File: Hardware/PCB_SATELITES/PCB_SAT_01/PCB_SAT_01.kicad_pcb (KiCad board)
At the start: 4 copper layers, 60 x 79 mm, 17 parts, among them IC1 OPT3001DNPRQ1, IC2 OPT3001DNPRQ1, IC3 OPT3001DNPRQ1, IC4 OPT3001DNPRQ1, J1 MTJ-88ARX1-FSM-LG

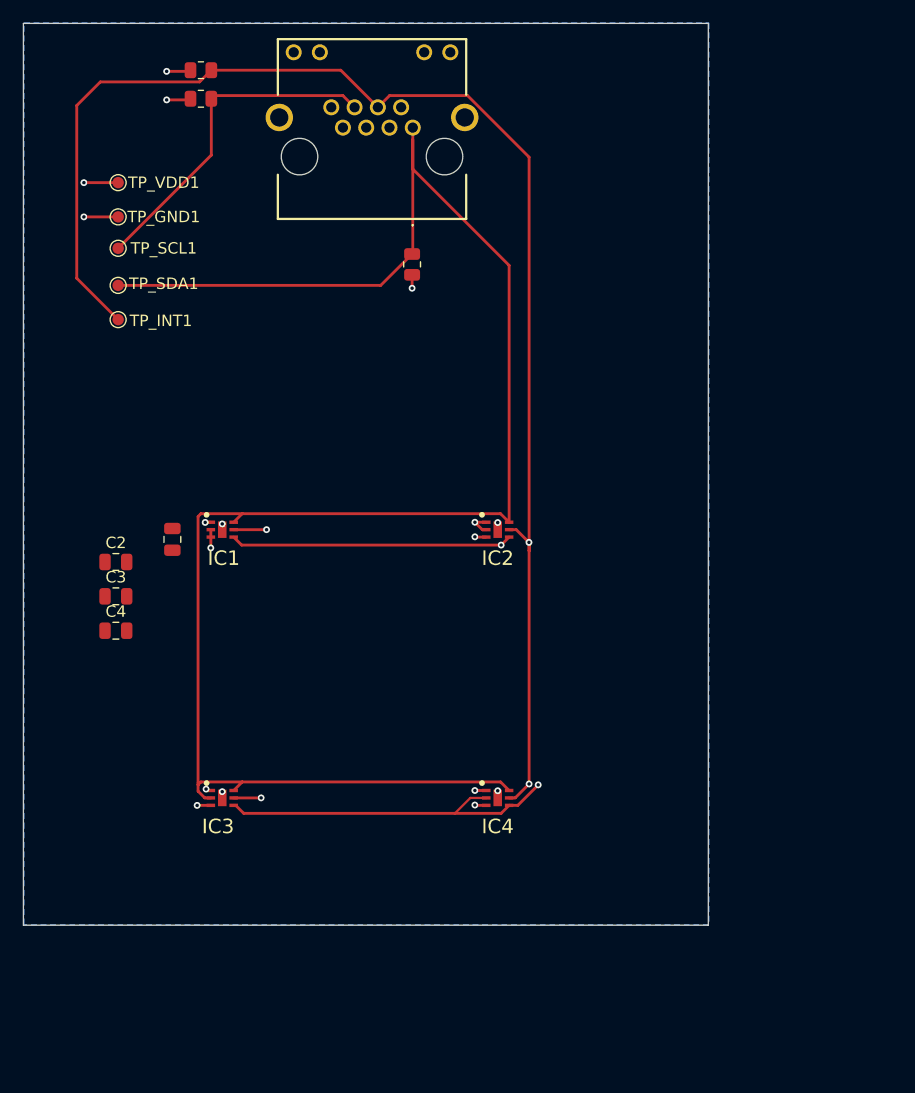
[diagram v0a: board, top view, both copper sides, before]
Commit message: actualizacion pcb satelite 1
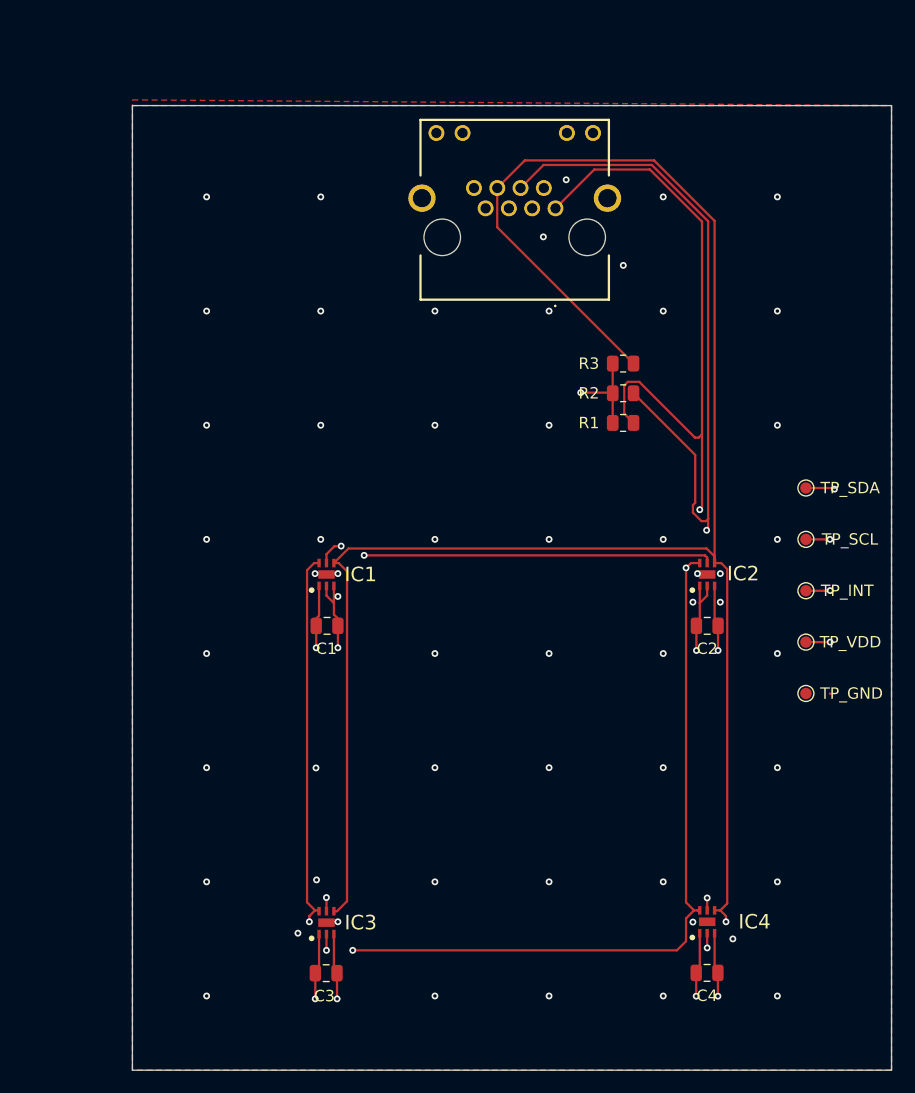
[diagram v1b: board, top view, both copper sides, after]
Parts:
- removed TP_GND1, TP_INT1, TP_SCL1, TP_SDA1, TP_VDD1: TestPoint, TestPoint:TestPoint_Pad_D1.0mm
- added TP_GND: TestPoint, TestPoint:TestPoint_Pad_D1.0mm, F.Cu at (142.5, 108.5)
- added TP_INT: TestPoint, TestPoint:TestPoint_Pad_D1.0mm, F.Cu at (142.5, 99.5)
- added TP_SCL: TestPoint, TestPoint:TestPoint_Pad_D1.0mm, F.Cu at (142.5, 95.0)
- added TP_SDA: TestPoint, TestPoint:TestPoint_Pad_D1.0mm, F.Cu at (142.5, 90.5)
- added TP_VDD: TestPoint, TestPoint:TestPoint_Pad_D1.0mm, F.Cu at (142.5, 104.0)
- moved C4 59.8 mm to (133.8, 133.0)
- moved C2 52.1 mm to (133.9, 102.6)
- moved R2 46.6 mm to (126.5, 82.2)
- moved R3 43.7 mm to (126.5, 79.6)
- moved C3 37.8 mm to (100.5, 133.0)
- moved R1 23.1 mm to (126.5, 84.8), turned to 0 degrees
- moved IC4 21.3 mm to (133.8, 128.5), turned to 90 degrees
- moved IC2 18.8 mm to (133.8, 98.1), turned to 90 degrees
- moved C1 15.5 mm to (100.5, 102.6), turned to 0 degrees
- moved J1 14.4 mm to (120.6, 66.0)
- moved IC3 14.2 mm to (100.5, 128.6), turned to 90 degrees
- moved IC1 9.94 mm to (100.5, 98.1), turned to 90 degrees
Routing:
- net /SCL: track 160.9 -> 221.8 mm, vias 2 -> 3
- net /INT: track 177.9 -> 232.2 mm, vias 4 -> 6
- net /SDA: track 158.3 -> 181.2 mm, vias 0 -> 6
- net VDD: track 12.7 -> 34.2 mm, vias 8 -> 6
- net GND: track 10.1 -> 24.0 mm, vias 9 -> 61
- added copper zone on In1.Cu, net (none)
- added copper zone on F.Cu, net GND
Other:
- board size 60 x 79 mm -> 66.5 x 84.5 mm
- board text removed: "OPT3001DNPRQ1"
- board text removed: "PCB SATELITE"
